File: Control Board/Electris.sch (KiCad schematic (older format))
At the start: 104 parts, among them J1 USB, J2 USB_BOOT, J3 SWD, J4 AUDIO, J5 VGA, J6 LED_1, Q1 MMBT2222ALT3G, SW1 SW_ML, SW2 SW_MR, SW3 SW_TL, SW4 SW_TR, SW5 SW_DS, SW6 SW_DH, SW7 SW_HL, U1 NCP1117LP-3.3_SOT223, U2 RP2040, U3 74LVC1G17, U4 74LVC1G17, U5 W25Q128JVS, U6 BCR401UW6Q, Y1 12MHz

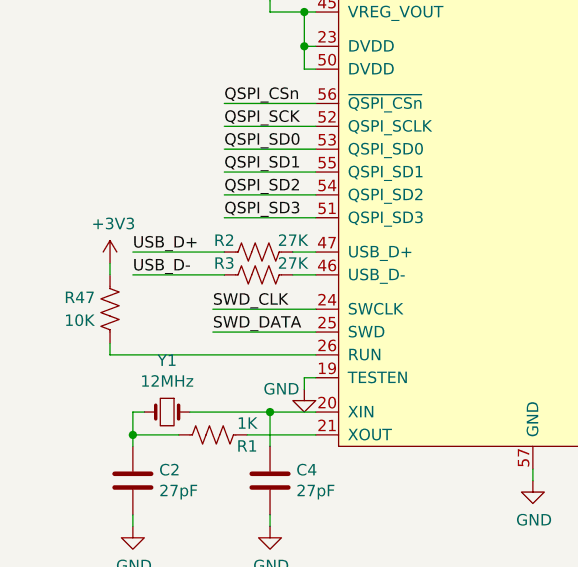
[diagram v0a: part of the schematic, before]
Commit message: Routing
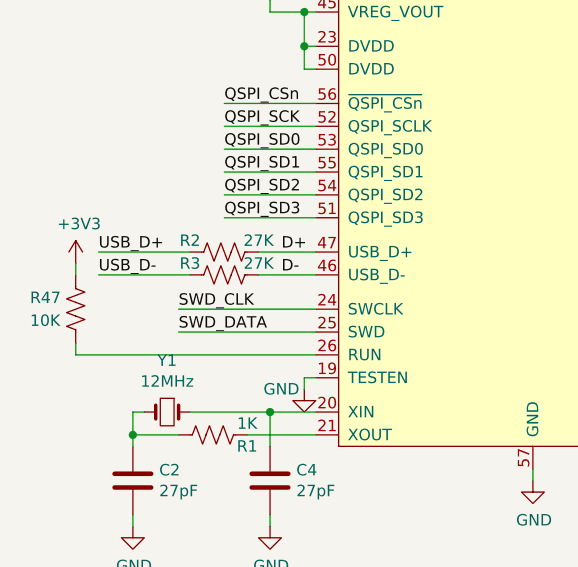
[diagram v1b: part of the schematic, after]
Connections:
- net D-: now reaches R3.1, U2.46 (USB_D-)
- net D+: now reaches R2.1, U2.47 (USB_D+)
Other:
- moved on the sheet: R2, R3, R47
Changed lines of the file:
@@
 Text Label 7150 2450 1    50   ~ 0
 AUDIO_R
-Text Label 1450 5200 0    50   ~ 0
+Text Label 1300 5200 0    50   ~ 0
 SWD_CLK
 Wire Wire Line
-	1450 5200 1900 5200
-Wire Wire Line
-	1450 5300 1900 5300
-Text Label 1450 5300 0    50   ~ 0
+	1300 5200 1900 5200
+Wire Wire Line
+	1300 5300 1900 5300
+Text Label 1300 5300 0    50   ~ 0
 SWD_DATA
 $Comp
@@
 L Device:R_US R2
 U 1 1 614243B8
-P 1650 4950
-F 0 "R2" V 1600 4800 50  0000 C CNN
-F 1 "27K" V 1600 5100 50  0000 C CNN
-F 2 "Resistor_SMD:R_0805_2012Metric_Pad1.20x1.40mm_HandSolder" V 1690 4940 50  0001 C CNN
-F 3 "~" H 1650 4950 50  0001 C CNN
-	1    1650 4950
-	0    1    1    0
-$EndComp
-Wire Wire Line
-	1800 4950 1900 4950
-Wire Wire Line
-	1900 5050 1800 5050
+P 1500 4950
+F 0 "R2" V 1450 4800 50  0000 C CNN
+F 1 "27K" V 1450 5100 50  0000 C CNN
+F 2 "Resistor_SMD:R_0805_2012Metric_Pad1.20x1.40mm_HandSolder" V 1540 4940 50  0001 C CNN
+F 3 "~" H 1500 4950 50  0001 C CNN
+	1    1500 4950
+	0    1    1    0
+$EndComp
+Wire Wire Line
+	1650 4950 1900 4950
+Wire Wire Line
+	1900 5050 1650 5050
 $Comp
 L Device:R_US R3
 U 1 1 61459653
-P 1650 5050
-F 0 "R3" V 1600 4900 50  0000 C CNN
-F 1 "27K" V 1600 5200 50  0000 C CNN
-F 2 "Resistor_SMD:R_0805_2012Metric_Pad1.20x1.40mm_HandSolder" V 1690 5040 50  0001 C CNN
-F 3 "~" H 1650 5050 50  0001 C CNN
-	1    1650 5050
-	0    1    1    0
-$EndComp
-Wire Wire Line
-	1500 4950 1100 4950
-Wire Wire Line
-	1100 5050 1500 5050
-Text Label 1100 4950 0    50   ~ 0
+P 1500 5050
+F 0 "R3" V 1450 4900 50  0000 C CNN
+F 1 "27K" V 1450 5200 50  0000 C CNN
+F 2 "Resistor_SMD:R_0805_2012Metric_Pad1.20x1.40mm_HandSolder" V 1540 5040 50  0001 C CNN
+F 3 "~" H 1500 5050 50  0001 C CNN
+	1    1500 5050
+	0    1    1    0
+$EndComp
+Wire Wire Line
+	1350 4950 950  4950
+Wire Wire Line
+	950  5050 1350 5050
+Text Label 950  4950 0    50   ~ 0
 USB_D+
-Text Label 1100 5050 0    50   ~ 0
+Text Label 950  5050 0    50   ~ 0
 USB_D-
 $Comp
@@
 L Device:R_US R47
 U 1 1 61BCC099
-P 1000 5200
-F 0 "R47" H 800 5250 50  0000 L CNN
-F 1 "10K" H 800 5150 50  0000 L CNN
-F 2 "Resistor_SMD:R_0603_1608Metric_Pad0.98x0.95mm_HandSolder" V 1040 5190 50  0001 C CNN
-F 3 "~" H 1000 5200 50  0001 C CNN
-	1    1000 5200
-	1    0    0    -1
-$EndComp
-Wire Wire Line
-	1900 5400 1000 5400
-Wire Wire Line
-	1000 5400 1000 5350
-Wire Wire Line
-	1000 5050 1000 5000
+P 850 5200
+F 0 "R47" H 650 5250 50  0000 L CNN
+F 1 "10K" H 650 5150 50  0000 L CNN
+F 2 "Resistor_SMD:R_0603_1608Metric_Pad0.98x0.95mm_HandSolder" V 890 5190 50  0001 C CNN
+F 3 "~" H 850 5200 50  0001 C CNN
+	1    850  5200
+	1    0    0    -1
+$EndComp
+Wire Wire Line
+	1900 5400 850  5400
+Wire Wire Line
+	850  5400 850  5350
+Wire Wire Line
+	850  5050 850  5000
 $Comp
 L power:+3V3 #PWR041
 U 1 1 61C8940C
-P 1000 5000
-F 0 "#PWR041" H 1000 4850 50  0001 C CNN
-F 1 "+3V3" H 1015 5173 50  0000 C CNN
-F 2 "" H 1000 5000 50  0001 C CNN
-F 3 "" H 1000 5000 50  0001 C CNN
-	1    1000 5000
-	1    0    0    -1
-$EndComp
+P 850 5000
+F 0 "#PWR041" H 850 4850 50  0001 C CNN
+F 1 "+3V3" H 865 5173 50  0000 C CNN
+F 2 "" H 850 5000 50  0001 C CNN
+F 3 "" H 850 5000 50  0001 C CNN
+	1    850  5000
+	1    0    0    -1
+$EndComp
+Text Label 1750 4950 0    50   ~ 0
+D+
+Text Label 1750 5050 0    50   ~ 0
+D-
 $EndSCHEMATC
